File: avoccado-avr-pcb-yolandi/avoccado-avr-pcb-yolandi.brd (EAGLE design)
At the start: 50 x 50 mm, 52 parts, among them Q1 16MHz, Q2 FET, U2 MCP73831

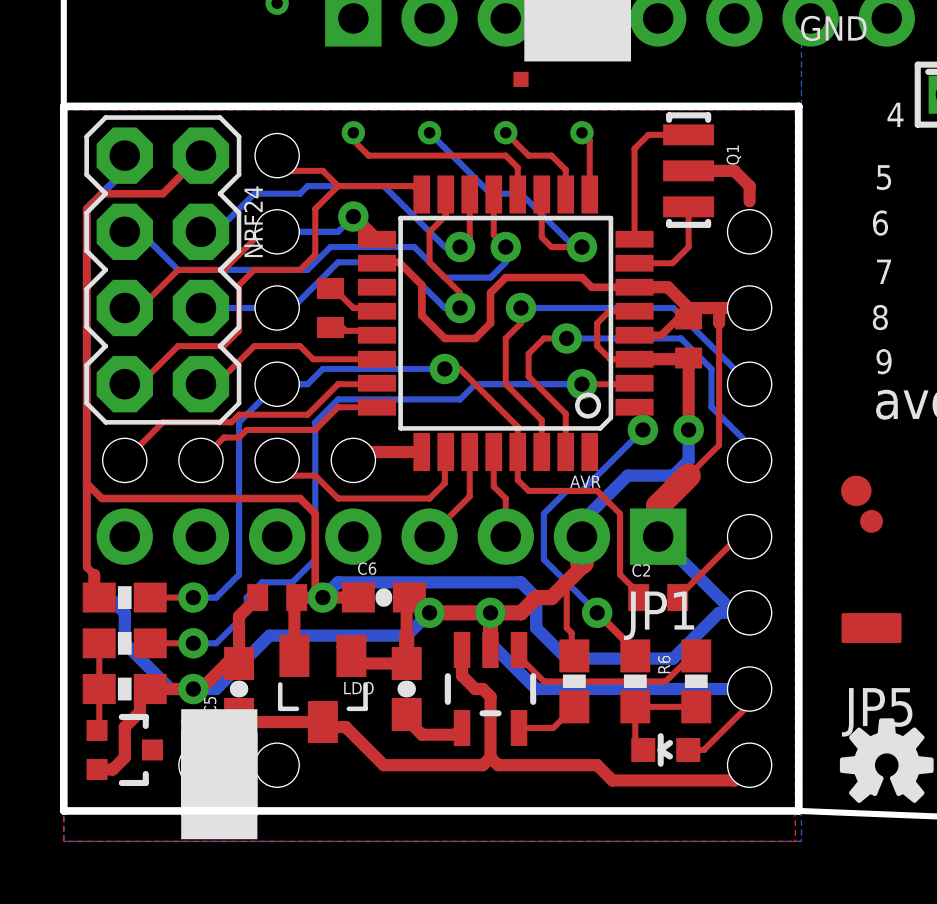
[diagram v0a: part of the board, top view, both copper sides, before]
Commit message: wip yolandi
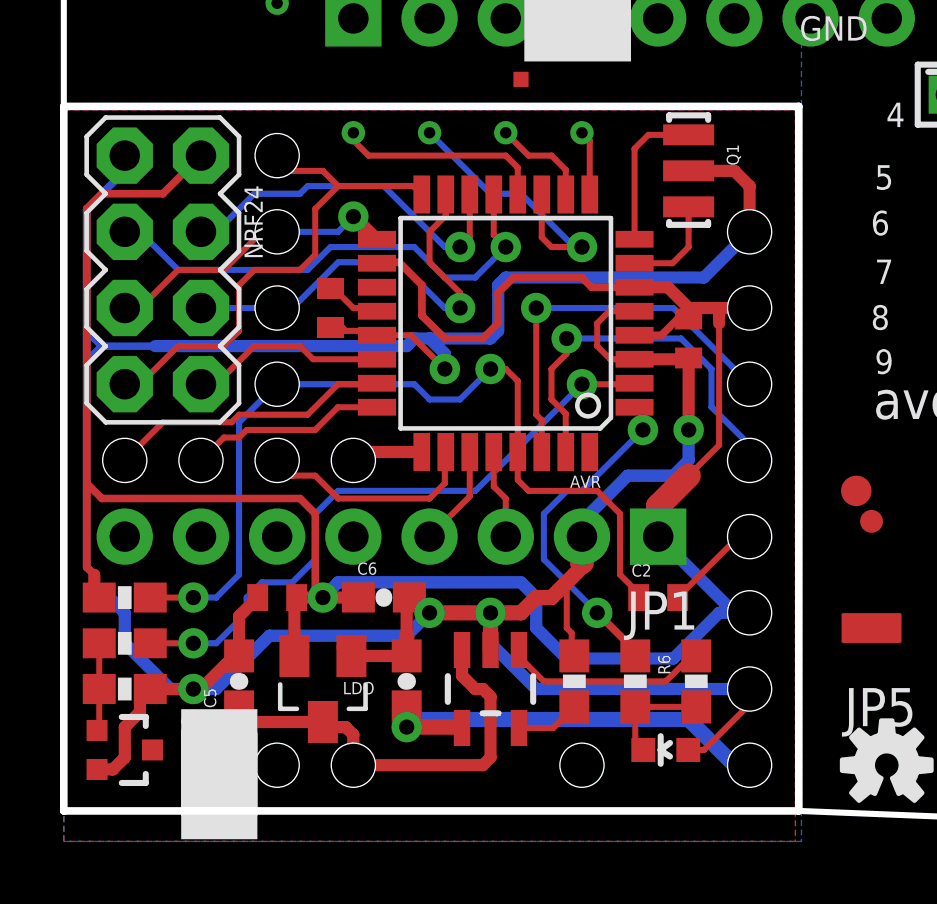
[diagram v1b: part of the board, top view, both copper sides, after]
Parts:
- added JP24: M01POGOPIN_HOLE_0.58, SparkFun-Connectors:1X01_POGOPIN_HOLE_0.58
- moved JP17 15.7 mm to (22.9, 2.54)
- moved JP7 13.2 mm to (9.65, 2.54)
- moved JP16 12.7 mm to (17.3, 2.54)
- moved C4 0.25 mm to (11.4, 5.33)
- moved C5 0.25 mm to (5.84, 5.33)
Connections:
- net GND: now also JP3.1
- net VBAT: now also JP24.1
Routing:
- net GND: track 89.7 -> 119.4 mm, vias 4 -> 5
- net 5V: track 2.31 -> 14.7 mm, vias 0 -> 1
- net VBAT: track 22.5 -> 14.1 mm
- net D4: track 22.7 -> 20.9 mm
- net RESET: track 27.9 -> 29.2 mm
- net RXI: track 14.2 -> 13.0 mm
- net TXO: track 14.1 -> 13.0 mm
